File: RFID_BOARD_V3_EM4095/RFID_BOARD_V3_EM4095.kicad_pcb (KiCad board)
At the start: 2 copper layers, 20 x 28.5 mm, 23 parts, among them J1 CONN_01X05, J2 CONN_01X01, J3 CONN_01X01, U1 EM4095

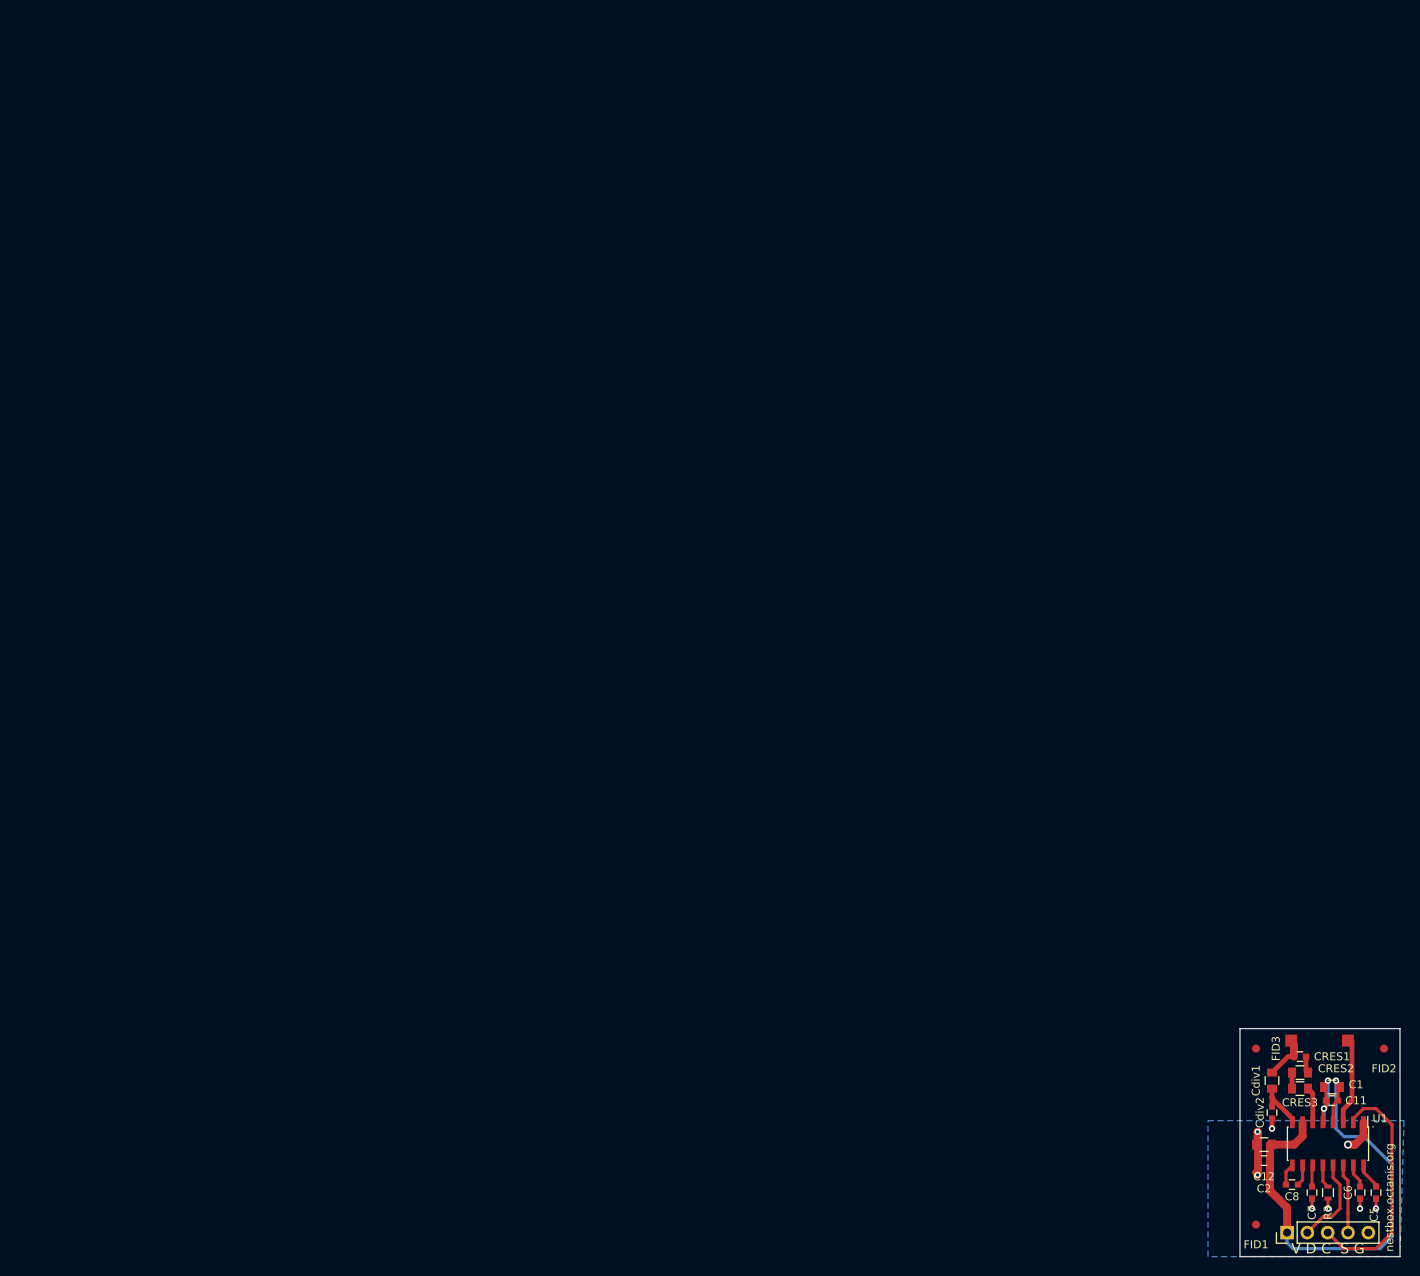
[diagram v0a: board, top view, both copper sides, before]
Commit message: various changes & updates, production state
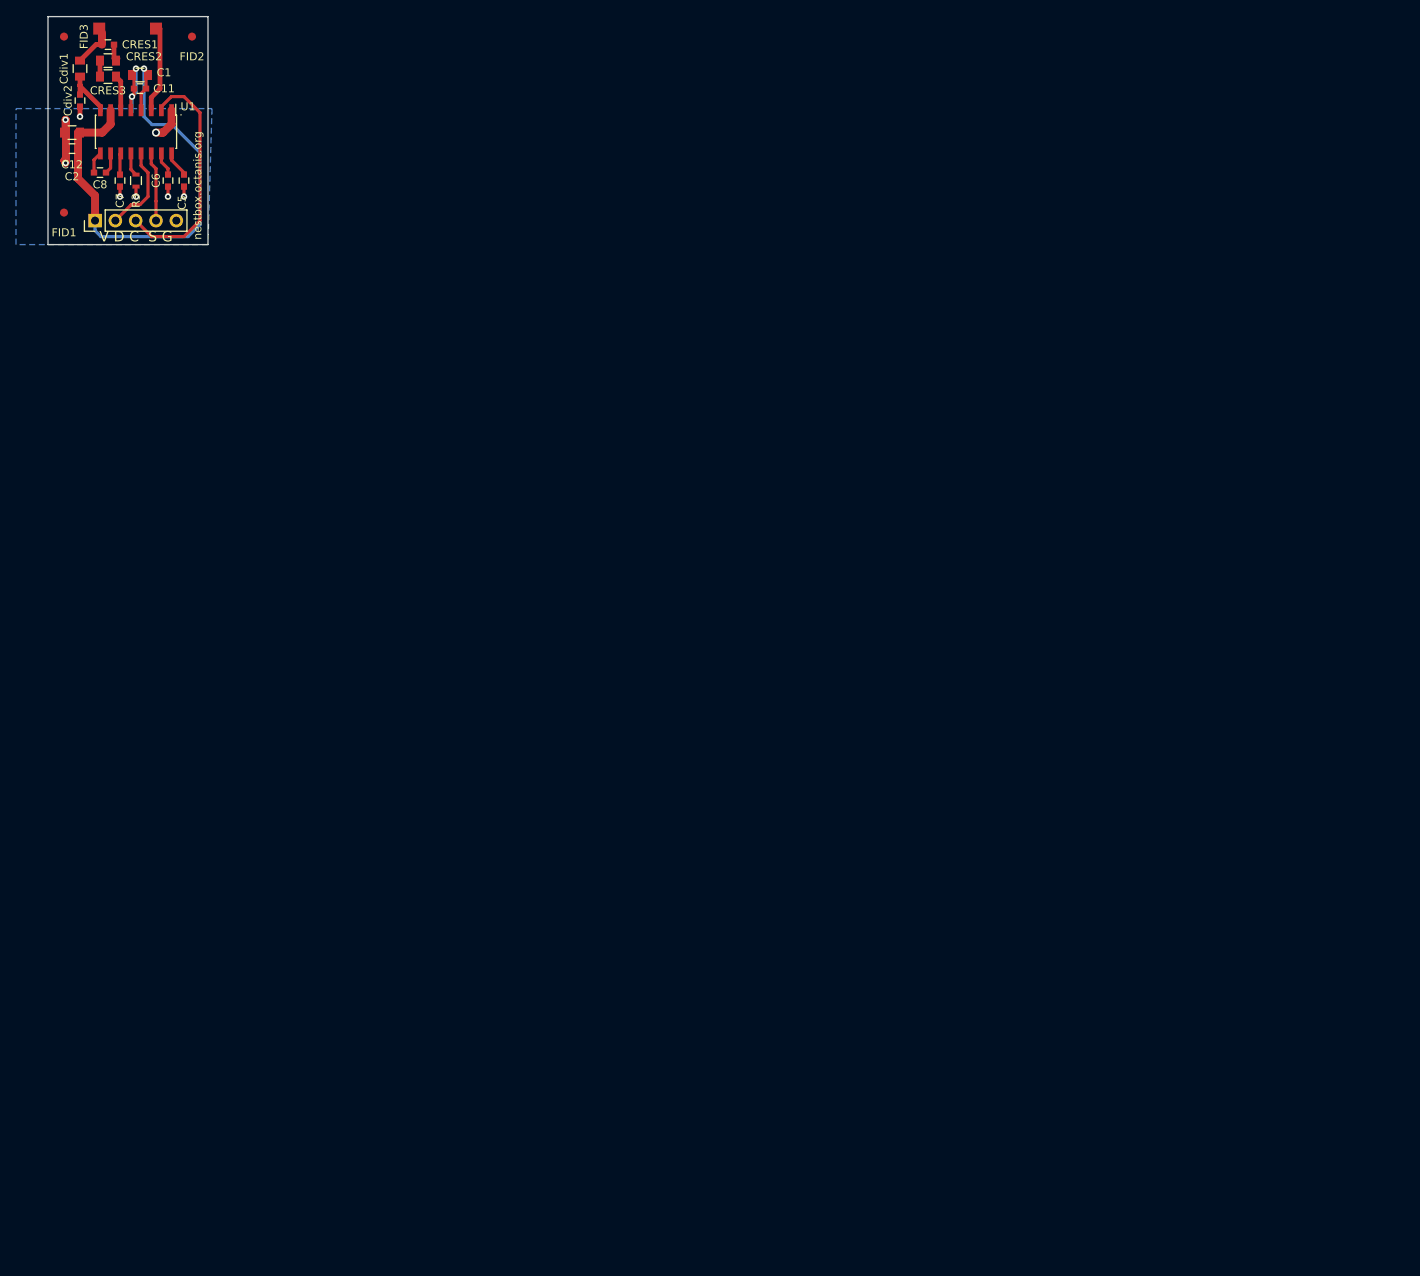
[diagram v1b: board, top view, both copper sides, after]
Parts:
- moved C1 195.5 mm to (11.5, -21.2)
- moved C11 195.5 mm to (11.5, -19.5)
- moved C12 195.5 mm to (3.00, -14.0)
- moved C2 195.5 mm to (3.00, -12.0)
- moved C5 195.5 mm to (17.0, -8.00)
- moved C6 195.5 mm to (15.0, -8.00)
- moved C7 195.5 mm to (9.00, -8.00)
- moved C8 195.5 mm to (6.50, -9.00)
- moved CRES1 195.5 mm to (7.50, -25.0)
- moved CRES2 195.5 mm to (7.50, -23.0)
- moved CRES3 195.5 mm to (7.50, -21.0)
- moved Cdiv1 195.5 mm to (4.00, -22.0)
- moved Cdiv2 195.5 mm to (4.00, -18.0)
- moved FID1 195.5 mm to (2.00, -4.00)
- moved FID2 195.5 mm to (18.0, -26.0)
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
